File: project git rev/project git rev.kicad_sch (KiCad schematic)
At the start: 31 parts, among them J1 Conn_01x03, J11 Conn_01x02, J4 Conn_01x02, J7 Conn_01x02, U1 LM358

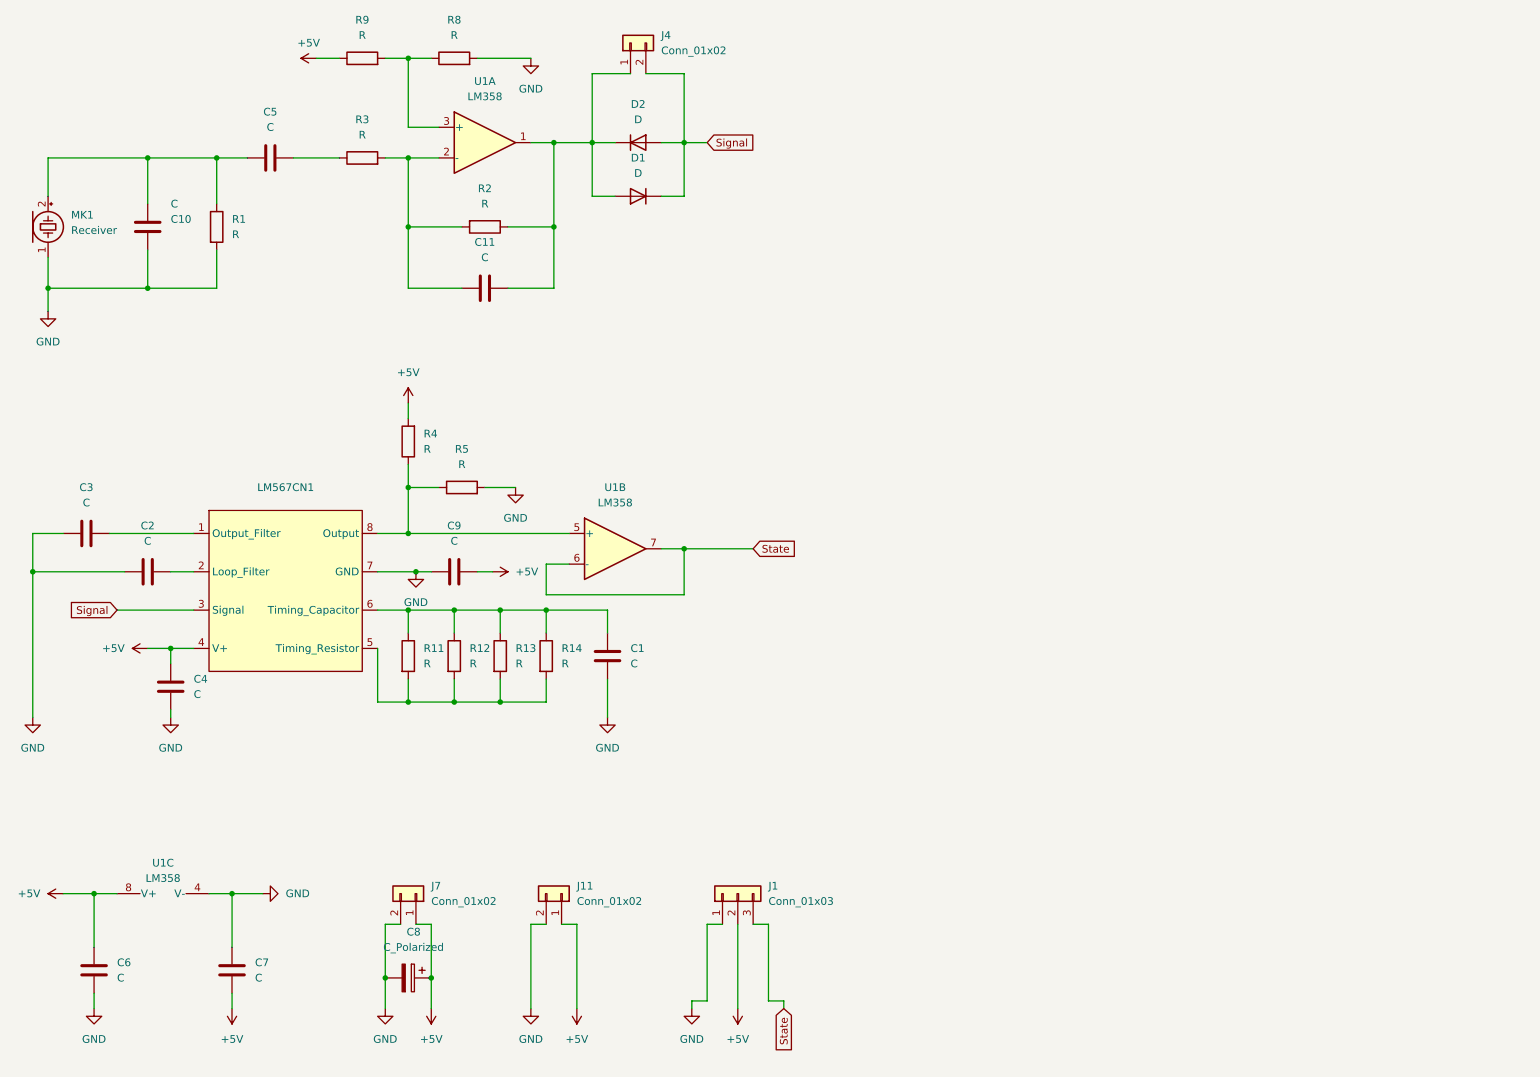
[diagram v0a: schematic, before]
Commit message: La til MCP adcen i kretsen og bestilte 👍
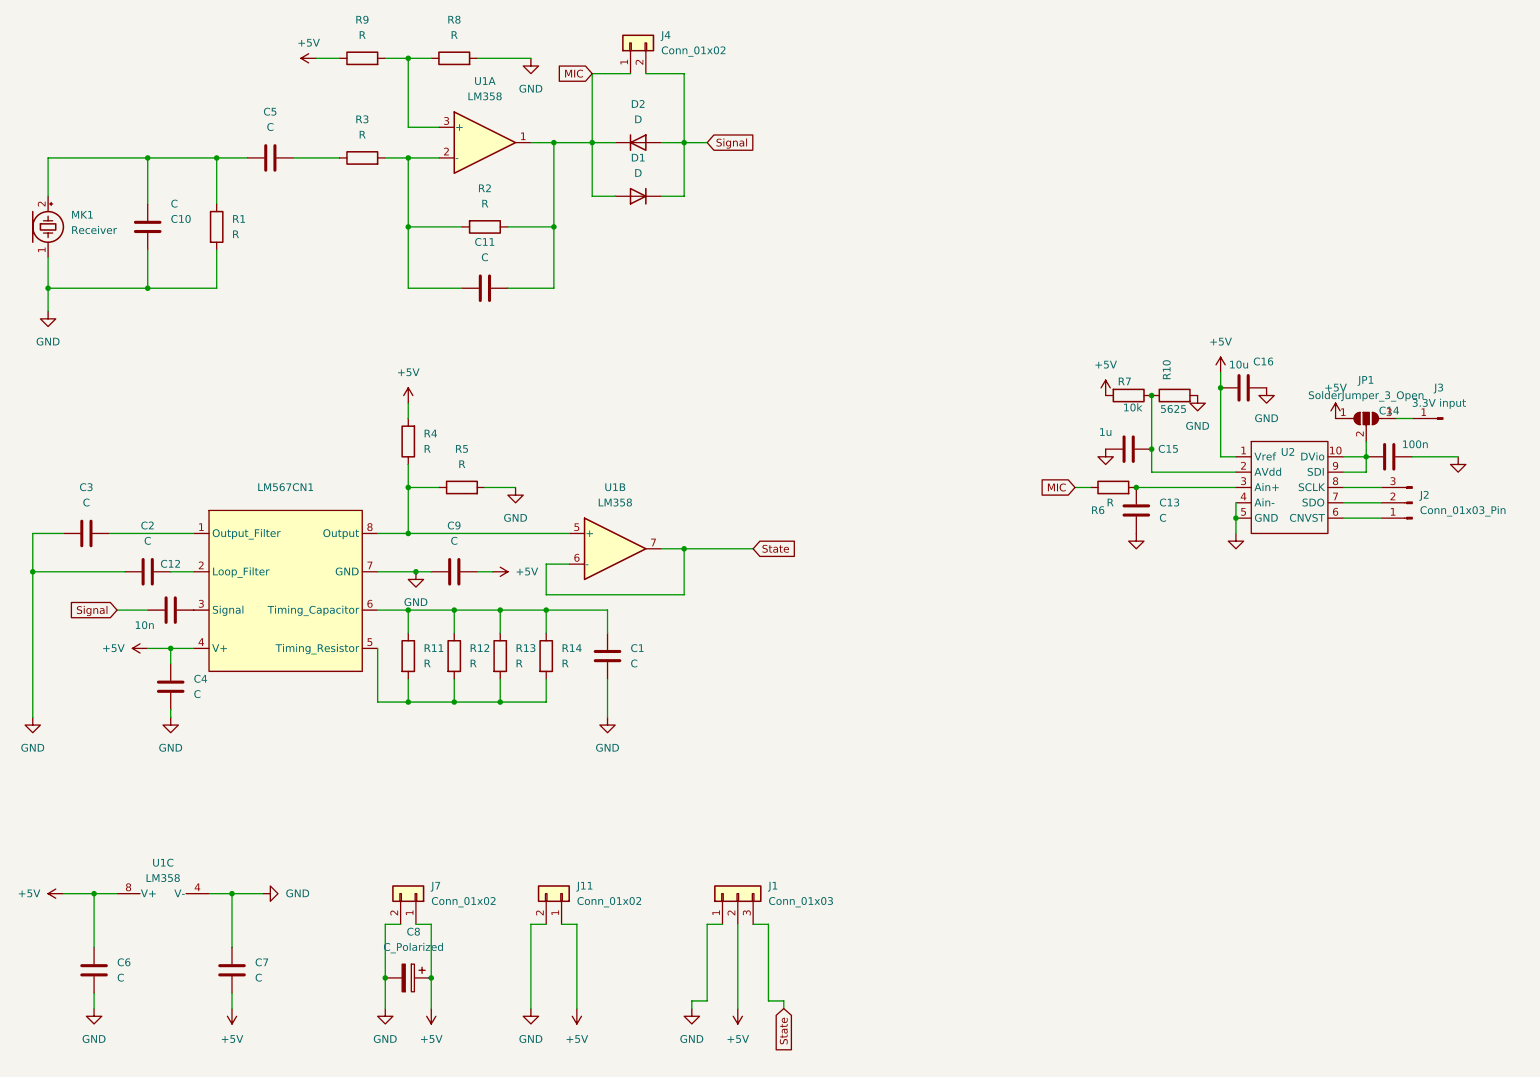
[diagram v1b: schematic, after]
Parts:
- added C12: 10n, UR:C_Rect_L4.6mm_W2.0mm_P2.50mm_MKS02_FKP02, symbol Device:C
- added C13: C, UR:C_Rect_L4.6mm_W2.0mm_P2.50mm_MKS02_FKP02, symbol Device:C
- added C14: 100n, UR:C_Rect_L4.6mm_W2.0mm_P2.50mm_MKS02_FKP02, symbol Device:C
- added C15: 1u, UR:C_Rect_L4.6mm_W2.0mm_P2.50mm_MKS02_FKP02, symbol Device:C
- added C16: 10u, UR:C_Rect_L4.6mm_W2.0mm_P2.50mm_MKS02_FKP02, symbol Device:C
- added J2: Conn_01x03_Pin, Connector_PinHeader_2.54mm:PinHeader_1x03_P2.54mm_Vertical, symbol Connector:Conn_01x03_Pin
- added J3: 3.3V input, Connector_PinHeader_2.54mm:PinHeader_1x01_P2.54mm_Vertical, symbol Connector:Conn_01x01_Pin
- added JP1: SolderJumper_3_Open, Jumper:SolderJumper-3_P2.0mm_Open_TrianglePad1.0x1.5mm, symbol Jumper:SolderJumper_3_Open
- added R10: 5625, UR:R_Axial_DIN0207_L6.3mm_D2.5mm_P10.16mm_Horizontal, symbol Device:R
- added R6: R, UR:R_Axial_DIN0207_L6.3mm_D2.5mm_P10.16mm_Horizontal, symbol Device:R
- added R7: 10k, UR:R_Axial_DIN0207_L6.3mm_D2.5mm_P10.16mm_Horizontal, symbol Device:R
- added U2: ~, Package_DFN_QFN:TDFN-10-1EP_2x3mm_P0.5mm_EP0.9x2mm, symbol Analog_ADC:MCP33151
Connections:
- net +5V: now also C16.1, JP1.1 (A), R7.2, U2.1 (Vref)
- net GND: now also C13.2, C14.2, C15.1, C16.2, R10.2, U2.4 (Ain-), U2.5 (GND)
- net Signal: now also C12.1; no longer LM567CN1.3 (Signal)
- net MIC: now reaches C11.2, D1.2 (A), D2.1 (K), J4.1 (Pin_1), R2.1, U1.1
- net MIC: now also R6.1
- new net: C13.1, R6.2, U2.3 (Ain+)
- new net: J3.1 (Pin_1), JP1.3 (B)
- new net: C14.1, JP1.2 (C), U2.10 (DVio), U2.9 (SDI)
- new net: C12.2, LM567CN1.3 (Signal)
- new net: C15.2, R10.1, R7.1, U2.2 (AVdd)
- new net: J2.1 (Pin_1), U2.6 (CNVST)
- new net: J2.2 (Pin_2), U2.7 (SDO)
- new net: J2.3 (Pin_3), U2.8 (SCLK)
